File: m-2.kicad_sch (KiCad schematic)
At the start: 26 parts, among them J2 1-2199230-6, Y1 ECS-327MVATX-2-CN-TR3

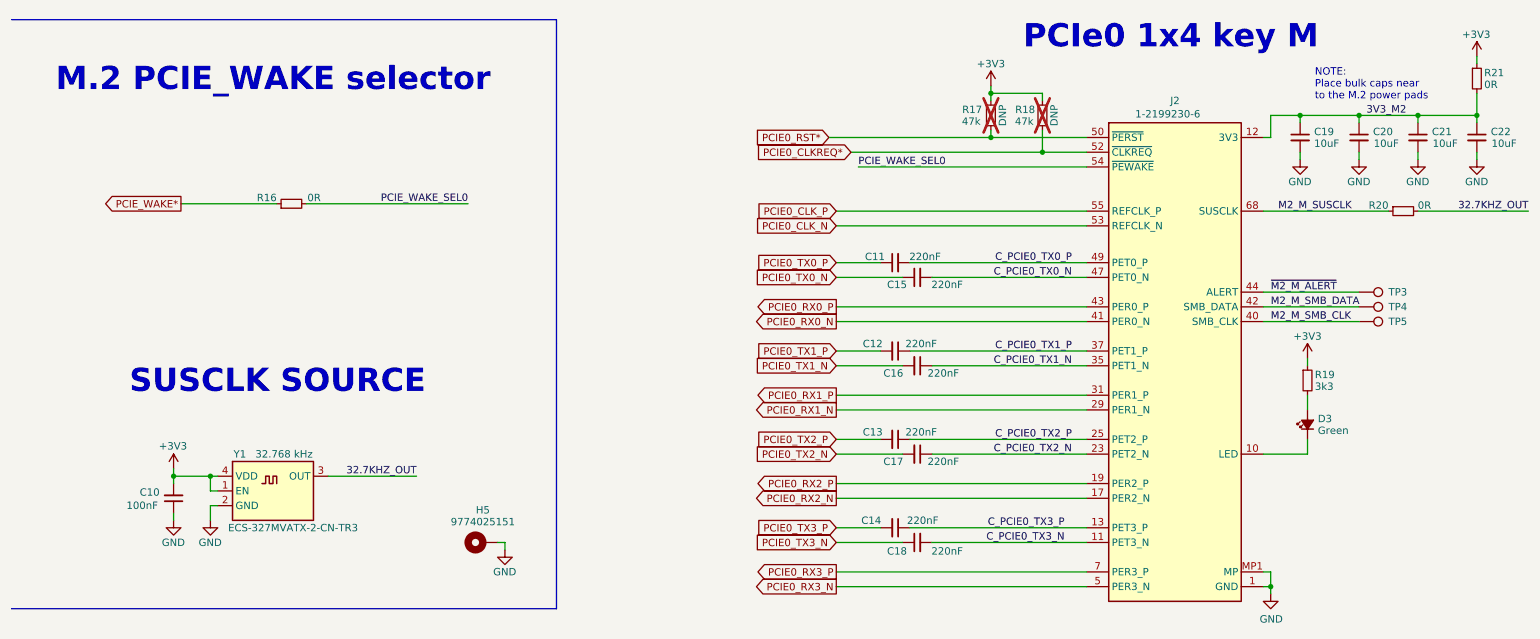
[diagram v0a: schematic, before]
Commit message: Final BOM changes, gerbers
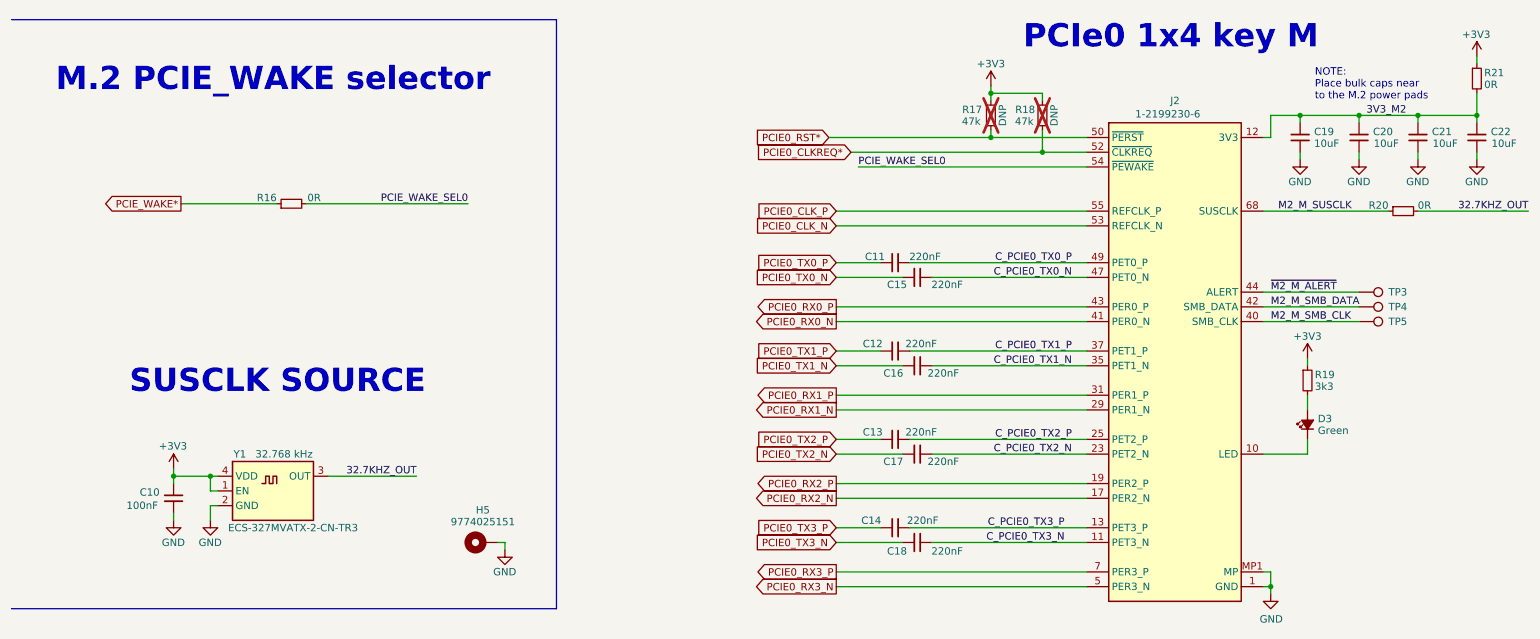
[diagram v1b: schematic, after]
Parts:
- C10: LCSC (none) -> C14663
- C11, C12, C13, C14, C15, C16, C17, C18: LCSC (none) -> C16772
- C19, C20, C21, C22: LCSC (none) -> C96446
- D3: LCSC (none) -> C12065
- J2: LCSC (none) -> C4710843
- R16, R20: LCSC (none) -> C17168
- R17, R18: LCSC (none) -> C25792
- R19: LCSC (none) -> C22978
- R21: LCSC (none) -> C21189
- Y1: LCSC (none) -> C5375606
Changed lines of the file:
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@@
 			)
 		)
+		(property "LCSC" "C5375606"
+			(at 52.07 151.13 0)
+			(effects
+				(font
+					(size 1.27 1.27)
+				)
+				(hide yes)
+			)
+		)
 		(pin "2"
 		)
@@
 			)
 		)
+		(property "LCSC" "C25792"
+			(at 189.23 92.456 0)
+			(effects
+				(font
+					(size 1.27 1.27)
+				)
+				(hide yes)
+			)
+		)
 		(pin "1"
 		)
@@
 			)
 		)
+		(property "LCSC" "C16772"
+			(at 159.512 132.842 0)
+			(effects
+				(font
+					(size 1.27 1.27)
+				)
+				(hide yes)
+			)
+		)
 		(pin "1"
 		)
@@
 			)
 		)
+		(property "LCSC" "C14663"
+			(at 34.798 156.972 0)
+			(effects
+				(font
+					(size 1.27 1.27)
+				)
+				(hide yes)
+			)
+		)
 		(pin "1"
 		)
@@
 			)
 		)
+		(property "LCSC" "C16772"
+			(at 167.132 121.158 0)
+			(effects
+				(font
+					(size 1.27 1.27)
+				)
+				(hide yes)
+			)
+		)
 		(pin "1"
 		)
@@
 			)
 		)
+		(property "LCSC" "C12065"
+			(at 237.998 145.034 0)
+			(effects
+				(font
+					(size 1.27 1.27)
+				)
+				(hide yes)
+			)
+		)
 		(pin "1"
 		)
@@
 			)
 		)
+		(property "LCSC" "C16772"
+			(at 159.512 148.082 0)
+			(effects
+				(font
+					(size 1.27 1.27)
+				)
+				(hide yes)
+			)
+		)
 		(pin "1"
 		)
@@
 			)
 		)
+		(property "LCSC" "C22978"
+			(at 237.49 138.176 0)
+			(effects
+				(font
+					(size 1.27 1.27)
+				)
+				(hide yes)
+			)
+		)
 		(pin "1"
 		)
@@
 			)
 		)
+		(property "LCSC" "C96446"
+			(at 261.112 96.266 0)
+			(effects
+				(font
+					(size 1.27 1.27)
+				)
+				(hide yes)
+			)
+		)
 		(pin "1"
 		)
@@
 			)
 		)
+		(property "LCSC" "C16772"
+			(at 163.068 137.922 0)
+			(effects
+				(font
+					(size 1.27 1.27)
+				)
+				(hide yes)
+			)
+		)
 		(pin "1"
 		)
@@
 			)
 		)
+		(property "LCSC" "C25792"
+			(at 180.086 92.456 0)
+			(effects
+				(font
+					(size 1.27 1.27)
+				)
+				(hide yes)
+			)
+		)
 		(pin "1"
 		)
@@
 			)
 		)
+		(property "LCSC" "C96446"
+			(at 250.952 96.266 0)
+			(effects
+				(font
+					(size 1.27 1.27)
+				)
+				(hide yes)
+			)
+		)
 		(pin "1"
 		)
@@
 			)
 		)
+		(property "LCSC" "C96446"
+			(at 271.272 96.266 0)
+			(effects
+				(font
+					(size 1.27 1.27)
+				)
+				(hide yes)
+			)
+		)
 		(pin "1"
 		)
@@
 			)
 		)
+		(property "LCSC" "C96446"
+			(at 240.792 96.266 0)
+			(effects
+				(font
+					(size 1.27 1.27)
+				)
+				(hide yes)
+			)
+		)
 		(pin "1"
 		)
@@
 			)
 		)
+		(property "LCSC" "C21189"
+			(at 266.7 86.106 0)
+			(effects
+				(font
+					(size 1.27 1.27)
+				)
+				(hide yes)
+			)
+		)
 		(pin "1"
 		)
@@
 			)
 		)
+		(property "LCSC" "C4710843"
+			(at 213.36 90.17 0)
+			(effects
+				(font
+					(size 1.27 1.27)
+				)
+				(hide yes)
+			)
+		)
 		(pin "1"
 		)
@@
 			)
 		)
+		(property "LCSC" "C17168"
+			(at 250.19 108.966 0)
+			(effects
+				(font
+					(size 1.27 1.27)
+				)
+				(hide yes)
+			)
+		)
 		(pin "1"
 		)
@@
 			)
 		)
+		(property "LCSC" "C16772"
+			(at 163.068 153.162 0)
+			(effects
+				(font
+					(size 1.27 1.27)
+				)
+				(hide yes)
+			)
+		)
 		(pin "1"
 		)
@@
 			)
 		)
+		(property "LCSC" "C17168"
+			(at 58.42 106.172 0)
+			(effects
+				(font
+					(size 1.27 1.27)
+				)
+				(hide yes)
+			)
+		)
 		(pin "1"
 		)
@@
 			)
 		)
+		(property "LCSC" "C16772"
+			(at 167.132 167.132 0)
+			(effects
+				(font
+					(size 1.27 1.27)
+				)
+				(hide yes)
+			)
+		)
 		(pin "1"
 		)
@@
 			)
 		)
+		(property "LCSC" "C16772"
+			(at 159.258 163.322 0)
+			(effects
+				(font
+					(size 1.27 1.27)
+				)
+				(hide yes)
+			)
+		)
 		(pin "1"
 		)
@@
 			)
 		)
+		(property "LCSC" "C16772"
+			(at 163.322 116.332 0)
+			(effects
+				(font
+					(size 1.27 1.27)
+				)
+				(hide yes)
+			)
+		)
